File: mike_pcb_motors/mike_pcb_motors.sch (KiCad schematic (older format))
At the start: 13 parts, among them J1 Motor1, J2 Motor2, J3 Motor3, J4 Motor1, J5 Screw_Terminal_01x02, J6 Motor2, J7 PCB_connector, U1 MDD3A-3ADCMD, U2 MDD3A-3ADCMD, U3 SBX-DRIVER, U5 DF_buck-converter_8-28to5V

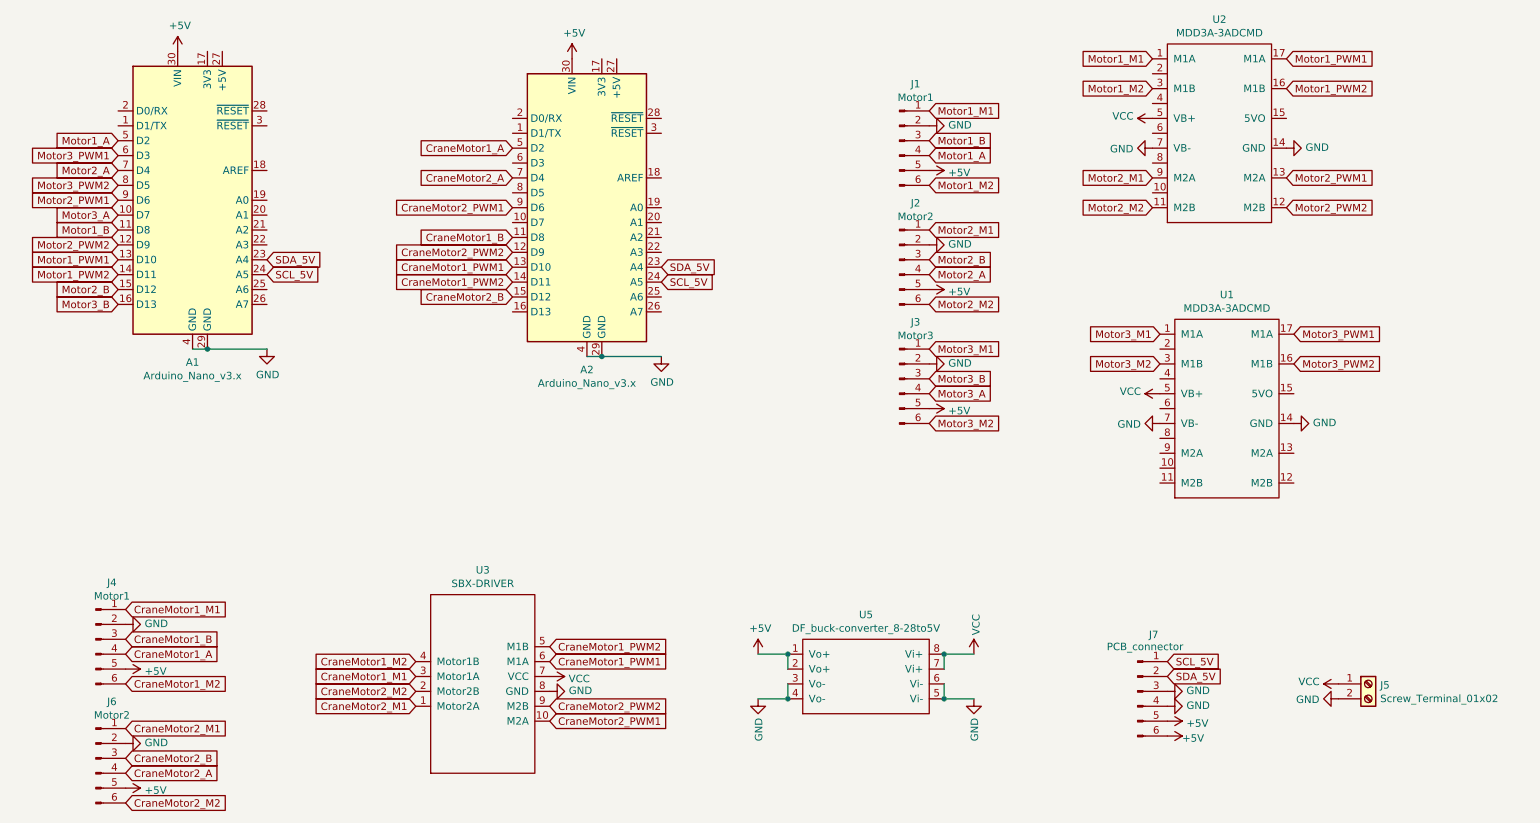
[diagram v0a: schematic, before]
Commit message: Updating the design files
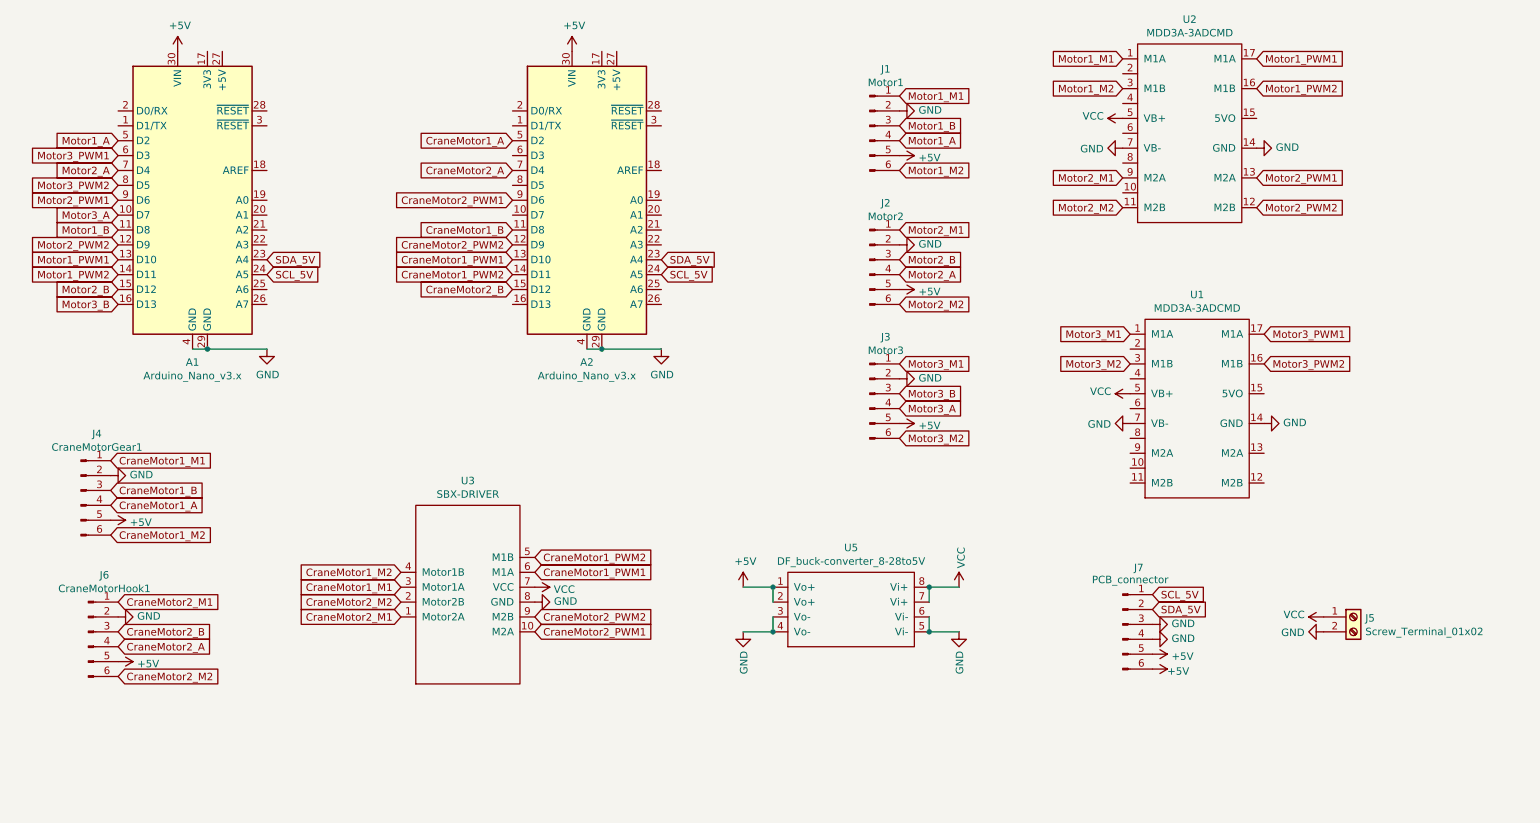
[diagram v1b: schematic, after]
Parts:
- J4: value Motor1 -> CraneMotorGear1
- J6: value Motor2 -> CraneMotorHook1
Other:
- moved on the sheet: A2, J1, J2, J3, J4, J5, J6, J7, U1, U2, U3, U5
